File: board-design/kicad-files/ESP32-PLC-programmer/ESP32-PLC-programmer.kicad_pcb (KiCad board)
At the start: 2 copper layers, 38.1 x 50.8 mm, 29 parts, among them J1 302-S101, J2 0473460001, J3 302-S101, U1 TPS62060DSGR, U2 FT231XS

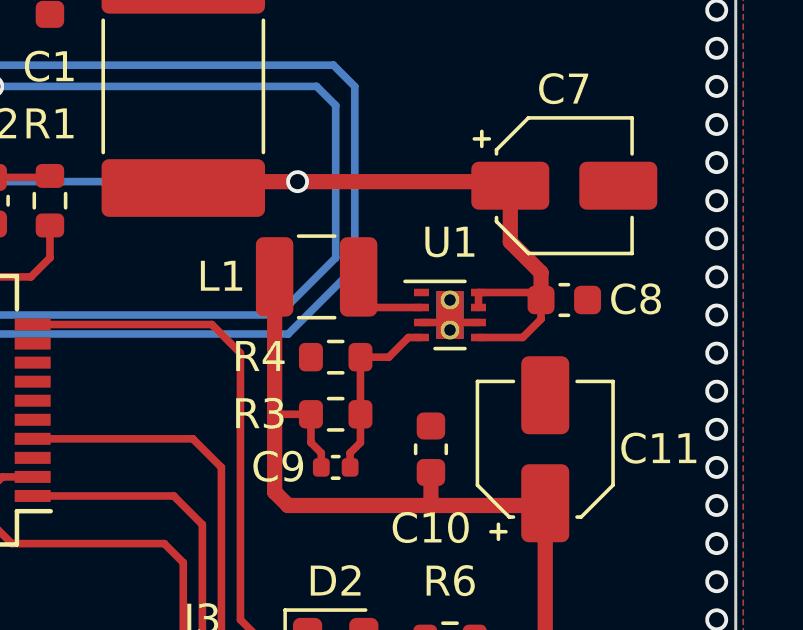
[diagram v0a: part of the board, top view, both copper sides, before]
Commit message: [Final report]
Added 3D models.

Signed-off-by: Nicolae-Andrei Vasile <vasilenicolaeandrei@gmail.com>
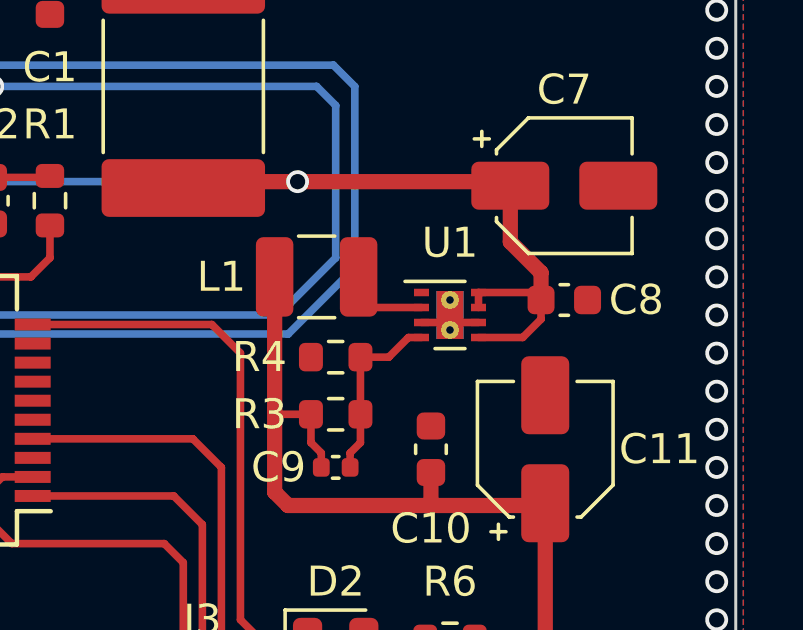
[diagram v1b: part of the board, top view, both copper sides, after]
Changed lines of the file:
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@@
     (pad "SH" smd rect (at 2.9125 0 270) (size 1.9 2.375) (layers "F.Cu" "F.Paste" "F.Mask")
       (net 13 "Earth_Protective") (pintype "passive"))
+    (model "${KIPRJMOD}/047346-0001.3dshapes/47346-0001.step"
+      (offset (xyz 0 0 1.27))
+      (scale (xyz 1 1 1))
+      (rotate (xyz 90 180 0))
+    )
   )
   (footprint "Capacitor_SMD:C_0603_1608Metric" (layer "F.Cu")
@@
     (property "ki_keywords" "diode Schottky")
     (attr smd)
-    (fp_text reference "D3" (at 0 -2.54 -180) (layer "F.SilkS")
+    (fp_text reference "D3" (at 0 -2.54) (layer "F.SilkS")
         (effects (font (size 1 1) (thickness 0.15)))
     )
@@
       (rotate (xyz 0 0 0))
     )
+    (model "/home/nick/Documents/Github/plc-embedded-application/board-design/kicad-files/libraries/kicad-packages3D-master/Diode_SMD.3dshapes/D_SOD-128.wrl"
+      (offset (xyz 0 0 0))
+      (scale (xyz 1 1 1))
+      (rotate (xyz 0 0 0))
+    )
   )
   (footprint "Capacitor_SMD:C_0603_1608Metric" (layer "F.Cu")
@@
     (property "ki_keywords" "fuse")
     (attr smd)
-    (fp_text reference "F1" (at -5.715 0 -180) (layer "F.SilkS")
+    (fp_text reference "F1" (at -5.715 0) (layer "F.SilkS")
         (effects (font (size 1 1) (thickness 0.15)))
     )
@@
       (net 5 "Net-(U1-AVIN)") (pintype "passive"))
     (model "${KICAD6_3DMODEL_DIR}/Fuse.3dshapes/Fuse_2920_7451Metric.wrl"
+      (offset (xyz 0 0 0))
+      (scale (xyz 1 1 1))
+      (rotate (xyz 0 0 0))
+    )
+    (model "/home/nick/Documents/Github/plc-embedded-application/board-design/kicad-files/libraries/kicad-packages3D-master/Resistor_SMD.3dshapes/R_2816_7142Metric.wrl"
       (offset (xyz 0 0 0))
       (scale (xyz 1 1 1))
@@
     (pad "8" smd rect (at 0.95 -0.75) (size 0.5 0.25) (layers "F.Cu" "F.Paste" "F.Mask")
       (net 5 "Net-(U1-AVIN)") (pinfunction "PVIN") (pintype "power_in"))
-    (pad "9" thru_hole circle (at 0 -0.5) (size 0.635 0.635) (drill 0.381) (layers "*.Cu"))
+    (pad "9" thru_hole circle (at 0 -0.5) (size 0.6 0.6) (drill 0.25) (layers "*.Cu"))
     (pad "9" smd rect (at 0 0) (size 0.9 1.6) (layers "F.Cu" "F.Mask"))
     (pad "9" smd rect (at 0 0) (size 0.9 1.6) (layers "B.Cu"))
-    (pad "9" thru_hole circle (at 0 0.5) (size 0.635 0.635) (drill 0.381) (layers "*.Cu"))
+    (pad "9" thru_hole circle (at 0 0.5) (size 0.6 0.6) (drill 0.25) (layers "*.Cu"))
     (model "${KICAD6_3DMODEL_DIR}/Package_SON.3dshapes/WSON-8-1EP_2x2mm_P0.5mm_EP0.9x1.6mm.wrl"
       (offset (xyz 0 0 0))
